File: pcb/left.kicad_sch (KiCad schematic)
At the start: 0 parts

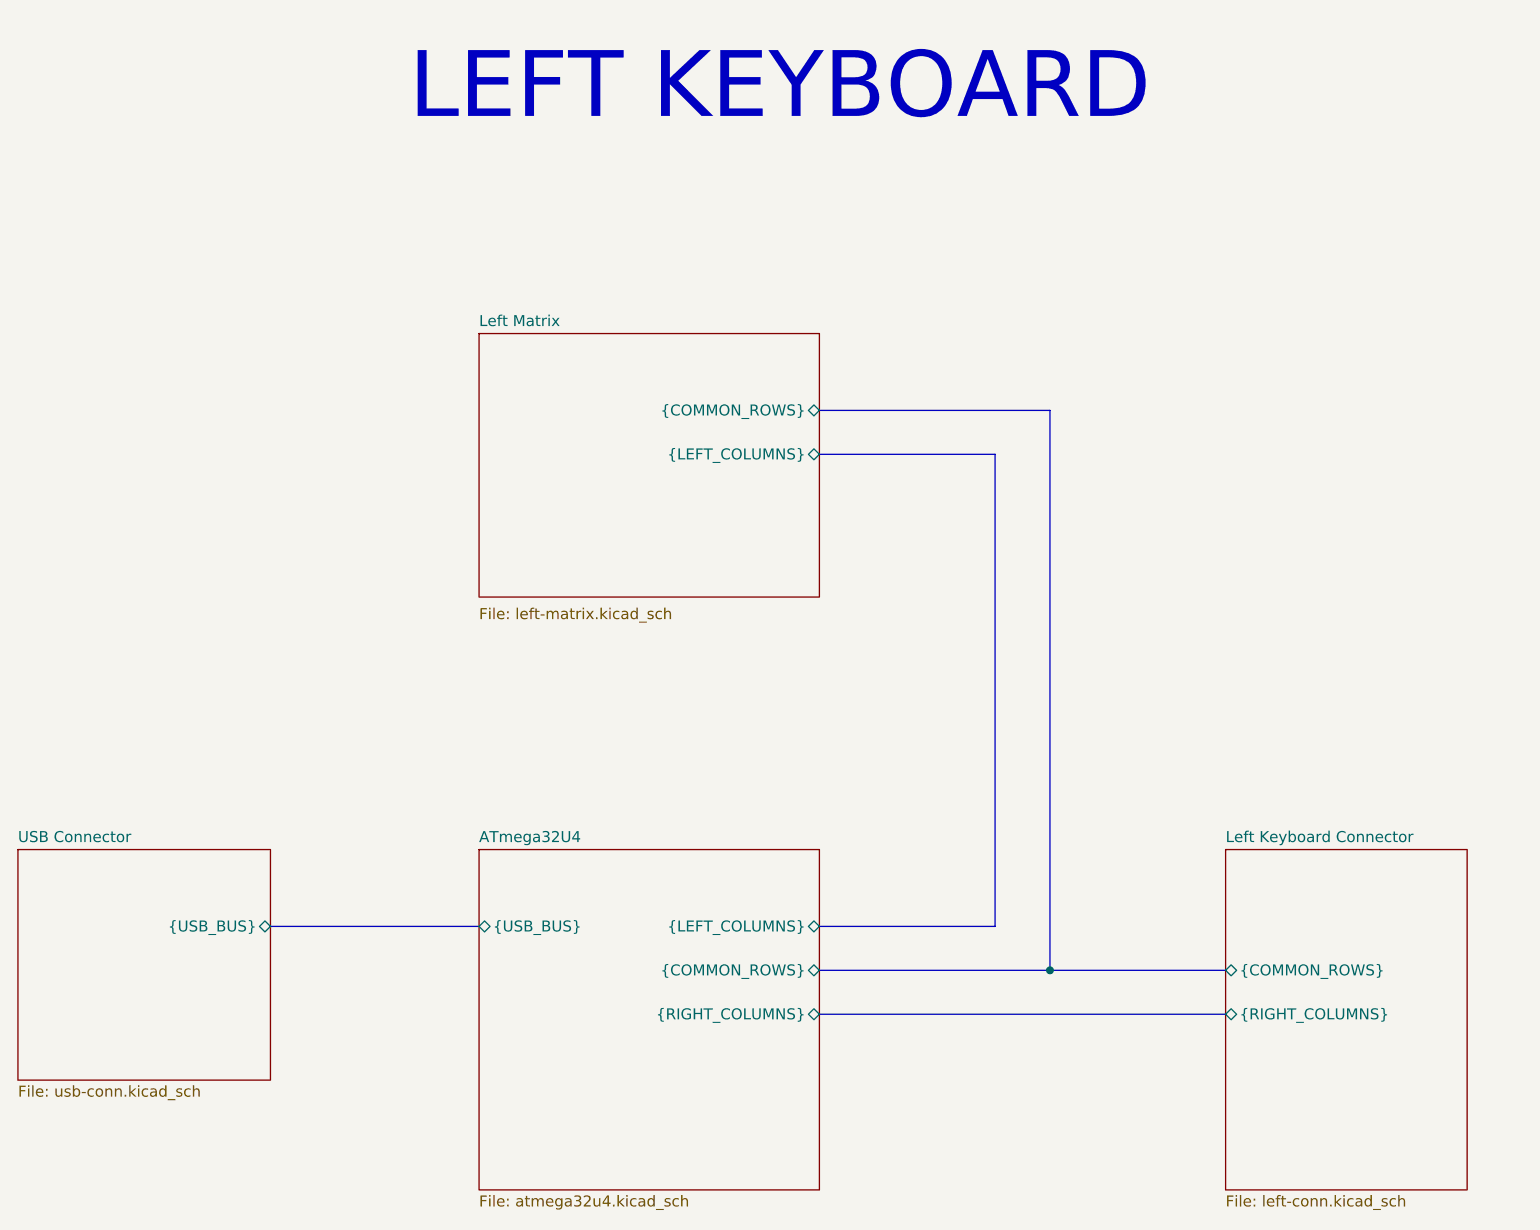
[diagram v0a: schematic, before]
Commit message: Continuing...no one will read this but me.
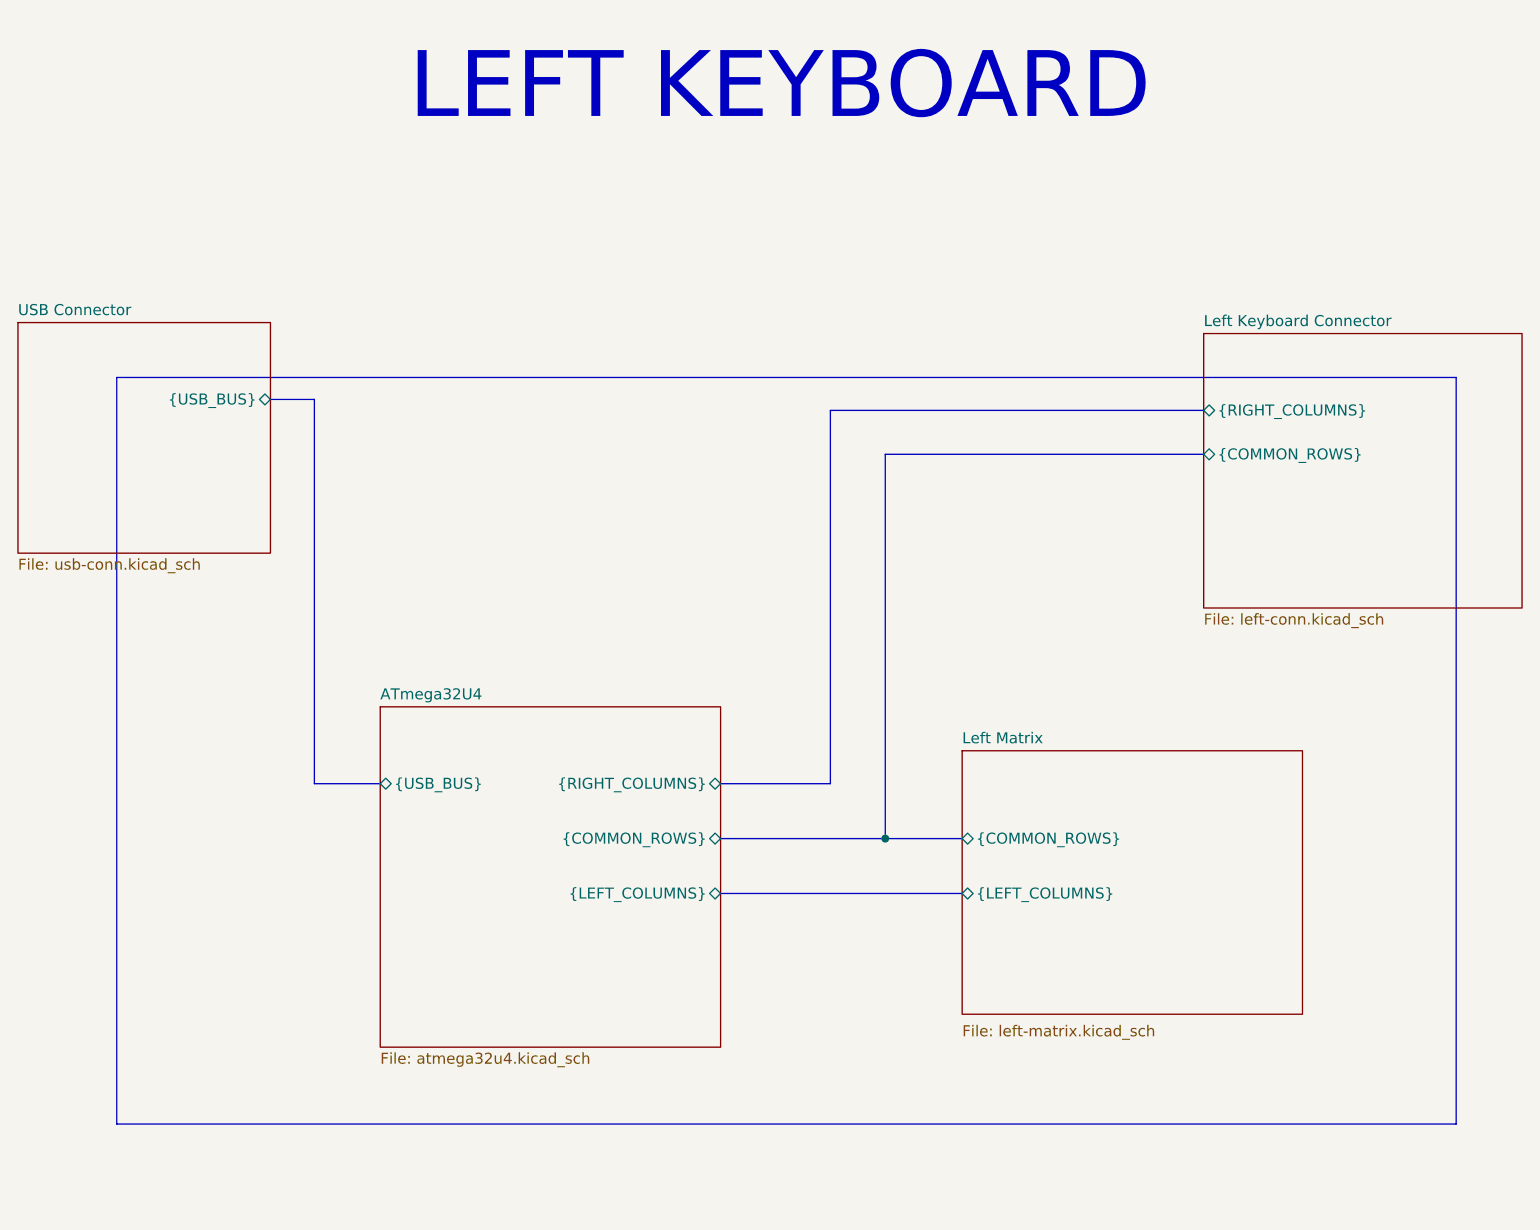
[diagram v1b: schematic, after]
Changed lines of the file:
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@@
 		(members "COL0" "COL1" "COL2" "COL3" "COL4" "COL5" "COL6")
+	)
+	(rectangle
+		(start 69.85 63.5)
+		(end 224.79 149.86)
+		(stroke
+			(width 0)
+			(type solid)
+			(color 255 43 5 1)
+		)
+		(fill
+			(type none)
+		)
 	)
 	(text "LEFT KEYBOARD"
@@
 	)
 	(junction
-		(at 177.8 132.08)
+		(at 158.75 116.84)
 		(diameter 0)
 		(color 0 0 0 0)
@@
 	(bus
 		(pts
-			(xy 177.8 132.08) (xy 177.8 67.31)
-		)
-		(stroke
-			(width 0)
-			(type default)
-		)
-	)
-	(bus
-		(pts
-			(xy 151.13 127) (xy 171.45 127)
-		)
-		(stroke
-			(width 0)
-			(type default)
-		)
-	)
-	(bus
-		(pts
-			(xy 151.13 137.16) (xy 198.12 137.16)
-		)
-		(stroke
-			(width 0)
-			(type default)
-		)
-	)
-	(bus
-		(pts
-			(xy 177.8 67.31) (xy 151.13 67.31)
-		)
-		(stroke
-			(width 0)
-			(type default)
-		)
-	)
-	(bus
-		(pts
-			(xy 151.13 132.08) (xy 177.8 132.08)
-		)
-		(stroke
-			(width 0)
-			(type default)
-		)
-	)
-	(bus
-		(pts
-			(xy 177.8 132.08) (xy 198.12 132.08)
-		)
-		(stroke
-			(width 0)
-			(type default)
-		)
-	)
-	(bus
-		(pts
-			(xy 87.63 127) (xy 111.76 127)
-		)
-		(stroke
-			(width 0)
-			(type default)
-		)
-	)
-	(bus
-		(pts
-			(xy 171.45 127) (xy 171.45 72.39)
-		)
-		(stroke
-			(width 0)
-			(type default)
-		)
-	)
-	(bus
-		(pts
-			(xy 151.13 72.39) (xy 171.45 72.39)
+			(xy 152.4 67.31) (xy 195.58 67.31)
+		)
+		(stroke
+			(width 0)
+			(type default)
+		)
+	)
+	(bus
+		(pts
+			(xy 139.7 116.84) (xy 158.75 116.84)
+		)
+		(stroke
+			(width 0)
+			(type default)
+		)
+	)
+	(bus
+		(pts
+			(xy 92.71 110.49) (xy 100.33 110.49)
+		)
+		(stroke
+			(width 0)
+			(type default)
+		)
+	)
+	(bus
+		(pts
+			(xy 92.71 66.04) (xy 92.71 110.49)
+		)
+		(stroke
+			(width 0)
+			(type default)
+		)
+	)
+	(bus
+		(pts
+			(xy 139.7 123.19) (xy 167.64 123.19)
+		)
+		(stroke
+			(width 0)
+			(type default)
+		)
+	)
+	(bus
+		(pts
+			(xy 152.4 67.31) (xy 152.4 110.49)
+		)
+		(stroke
+			(width 0)
+			(type default)
+		)
+	)
+	(bus
+		(pts
+			(xy 87.63 66.04) (xy 92.71 66.04)
+		)
+		(stroke
+			(width 0)
+			(type default)
+		)
+	)
+	(bus
+		(pts
+			(xy 158.75 72.39) (xy 158.75 116.84)
+		)
+		(stroke
+			(width 0)
+			(type default)
+		)
+	)
+	(bus
+		(pts
+			(xy 158.75 116.84) (xy 167.64 116.84)
+		)
+		(stroke
+			(width 0)
+			(type default)
+		)
+	)
+	(bus
+		(pts
+			(xy 139.7 110.49) (xy 152.4 110.49)
+		)
+		(stroke
+			(width 0)
+			(type default)
+		)
+	)
+	(bus
+		(pts
+			(xy 158.75 72.39) (xy 195.58 72.39)
 		)
 		(stroke
@@
 	)
 	(sheet
-		(at 111.76 58.42)
+		(at 167.64 106.68)
 		(size 39.37 30.48)
 		(exclude_from_sim no)
@@
 		)
 		(property "Sheetname" "Left Matrix"
-			(at 111.76 57.7084 0)
+			(at 167.64 105.9684 0)
 			(effects
 				(font
@@
 		)
 		(property "Sheetfile" "left-matrix.kicad_sch"
-			(at 111.76 90.1196 0)
+			(at 167.64 138.3796 0)
 			(effects
 				(font
@@
 		)
 		(pin "{COMMON_ROWS}" bidirectional
-			(at 151.13 67.31 0)
-			(effects
-				(font
-					(size 1.27 1.27)
-				)
-				(justify right)
+			(at 167.64 116.84 180)
+			(effects
+				(font
+					(size 1.27 1.27)
+				)
+				(justify left)
 			)
 		)
 		(pin "{LEFT_COLUMNS}" bidirectional
-			(at 151.13 72.39 0)
-			(effects
-				(font
-					(size 1.27 1.27)
-				)
-				(justify right)
+			(at 167.64 123.19 180)
+			(effects
+				(font
+					(size 1.27 1.27)
+				)
+				(justify left)
 			)
 		)
 		(instances
-			(project "split-normal-69"
+			(project "69split"
 				(path "/d75b0717-10e3-4e20-afcb-05300684210e/a528eaf3-d99a-4f91-978f-500370d04b37"
 					(page "7")
 				)
 			)
+			(project ""
+				(path "/619d845a-8c90-490b-ae7a-6c3e22416b6d"
+					(page "#")
+				)
+			)
+			(project "69split-left"
+				(path "/94301c1c-44b1-4926-ac38-8a25b84a2b23/619d845a-8c90-490b-ae7a-6c3e22416b6d"
+					(page "5")
+				)
+			)
 		)
 	)
 	(sheet
-		(at 111.76 118.11)
+		(at 100.33 101.6)
 		(size 39.37 39.37)
 		(exclude_from_sim no)
@@
 		)
 		(property "Sheetname" "ATmega32U4"
-			(at 111.76 117.3984 0)
+			(at 100.33 100.8884 0)
 			(effects
 				(font
@@
 		)
 		(property "Sheetfile" "atmega32u4.kicad_sch"
-			(at 111.76 158.0646 0)
+			(at 100.33 141.5546 0)
 			(effects
 				(font
@@
 		)
 		(pin "{COMMON_ROWS}" bidirectional
-			(at 151.13 132.08 0)
+			(at 139.7 116.84 0)
 			(effects
 				(font
@@
 		)
 		(pin "{LEFT_COLUMNS}" bidirectional
-			(at 151.13 127 0)
+			(at 139.7 123.19 0)
 			(effects
 				(font
@@
 		)
 		(pin "{RIGHT_COLUMNS}" bidirectional
-			(at 151.13 137.16 0)
+			(at 139.7 110.49 0)
 			(effects
 				(font
@@
 		)
 		(pin "{USB_BUS}" bidirectional
-			(at 111.76 127 180)
+			(at 100.33 110.49 180)
 			(effects
 				(font
@@
 		)
 		(instances
-			(project "split-normal-69"
+			(project "69split"
 				(path "/d75b0717-10e3-4e20-afcb-05300684210e/a528eaf3-d99a-4f91-978f-500370d04b37"
 					(page "6")
 				)
 			)
+			(project ""
+				(path "/619d845a-8c90-490b-ae7a-6c3e22416b6d"
+					(page "#")
+				)
+			)
+			(project "69split-left"
+				(path "/94301c1c-44b1-4926-ac38-8a25b84a2b23/619d845a-8c90-490b-ae7a-6c3e22416b6d"
+					(page "4")
+				)
+			)
 		)
 	)
 	(sheet
-		(at 58.42 118.11)
+		(at 58.42 57.15)
 		(size 29.21 26.67)
 		(exclude_from_sim no)
@@
 		)
 		(property "Sheetname" "USB Connector"
-			(at 58.42 117.3984 0)
+			(at 58.42 56.4384 0)
 			(effects
 				(font
@@
 		)
 		(property "Sheetfile" "usb-conn.kicad_sch"
-			(at 58.42 145.3646 0)
+			(at 58.42 84.4046 0)
 			(effects
 				(font
@@
 		)
 		(pin "{USB_BUS}" bidirectional
-			(at 87.63 127 0)
+			(at 87.63 66.04 0)
 			(effects
 				(font
@@
 		)
 		(instances
-			(project "split-normal-69"
+			(project "69split"
 				(path "/d75b0717-10e3-4e20-afcb-05300684210e/a528eaf3-d99a-4f91-978f-500370d04b37"
 					(page "8")
 				)
 			)
+			(project ""
+				(path "/619d845a-8c90-490b-ae7a-6c3e22416b6d"
+					(page "#")
+				)
+			)
+			(project "69split-left"
+				(path "/94301c1c-44b1-4926-ac38-8a25b84a2b23/619d845a-8c90-490b-ae7a-6c3e22416b6d"
+					(page "3")
+				)
+			)
 		)
 	)
 	(sheet
-		(at 198.12 118.11)
-		(size 27.94 39.37)
+		(at 195.58 58.42)
+		(size 36.83 31.75)
 		(exclude_from_sim no)
 		(in_bom yes)
@@
 		)
 		(property "Sheetname" "Left Keyboard Connector"
-			(at 198.12 117.3984 0)
+			(at 195.58 57.7084 0)
 			(effects
 				(font
@@
 		)
 		(property "Sheetfile" "left-conn.kicad_sch"
-			(at 198.12 158.0646 0)
+			(at 195.58 90.7546 0)
 			(effects
 				(font
@@
 		)
 		(pin "{COMMON_ROWS}" bidirectional
-			(at 198.12 132.08 180)
+			(at 195.58 72.39 180)
 			(effects
 				(font
@@
 		)
 		(pin "{RIGHT_COLUMNS}" bidirectional
-			(at 198.12 137.16 180)
+			(at 195.58 67.31 180)
 			(effects
 				(font
@@
 		)
 		(instances
-			(project "split-normal-69"
+			(project "69split"
 				(path "/d75b0717-10e3-4e20-afcb-05300684210e/a528eaf3-d99a-4f91-978f-500370d04b37"
 					(page "4")
 				)
 			)
+			(project ""
+				(path "/619d845a-8c90-490b-ae7a-6c3e22416b6d"
+					(page "#")
+				)
+			)
+			(project "69split-left"
+				(path "/94301c1c-44b1-4926-ac38-8a25b84a2b23/619d845a-8c90-490b-ae7a-6c3e22416b6d"
+					(page "6")
+				)
+			)
